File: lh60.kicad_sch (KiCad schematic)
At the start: 31 parts, among them J1 Conn_01x03_Female, J3 Conn_01x02_Female, J5 Conn_01x02_Female, P1 USB_C_Plug_USB2.0, SW1 SW_Push, U1 AMS1117-3.3, U2 STM32F103C8Tx, Y1 32.768K, Y2 8M

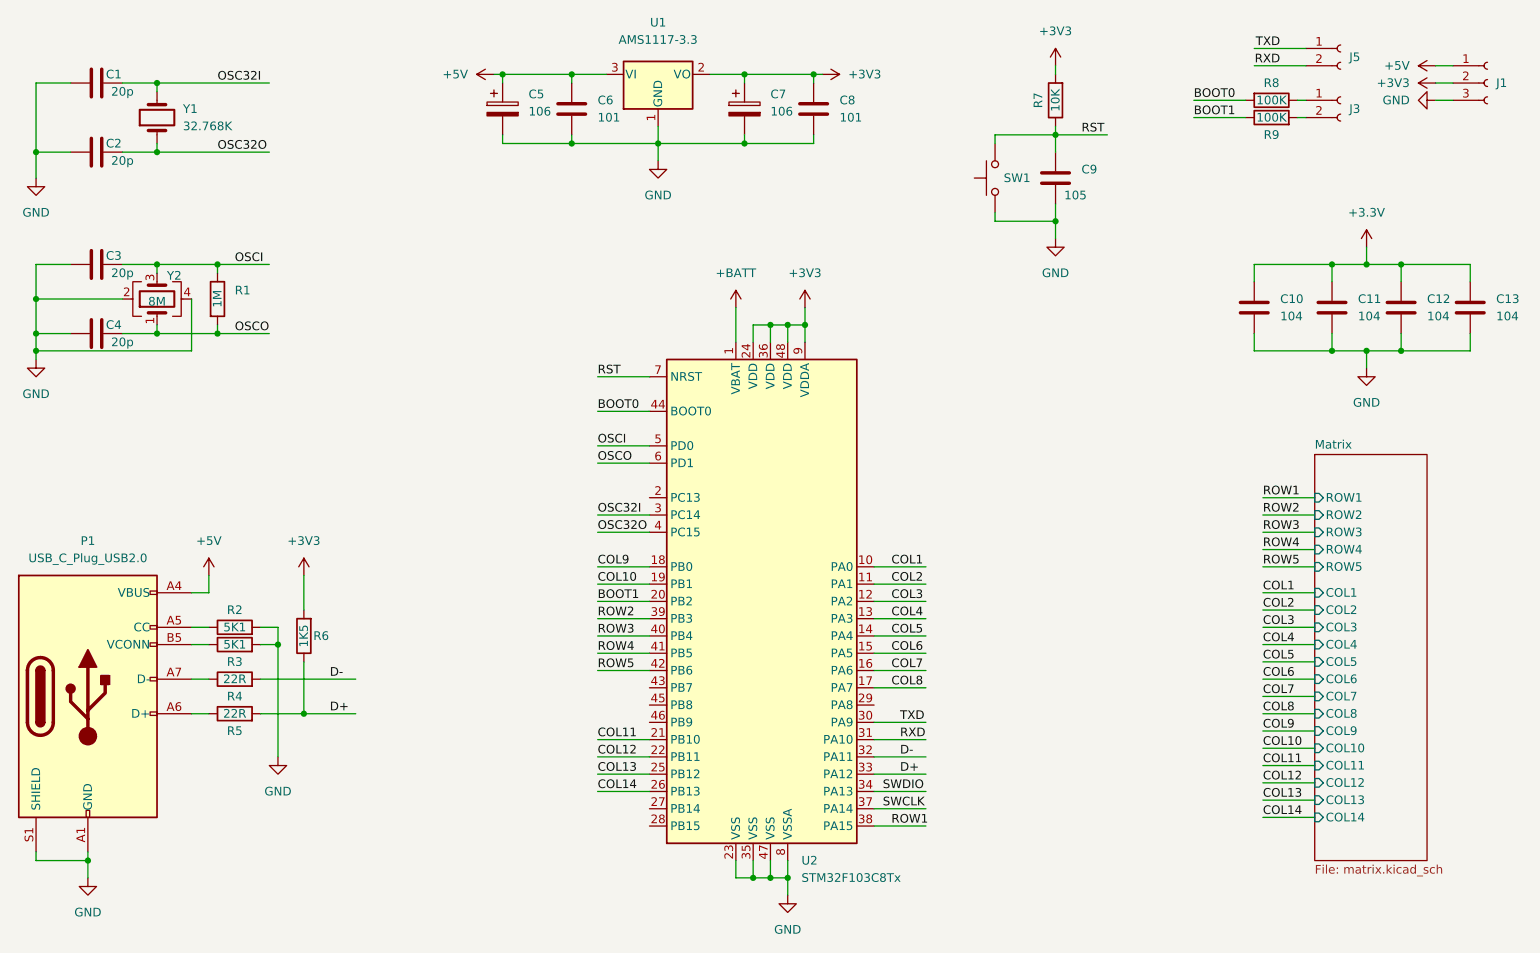
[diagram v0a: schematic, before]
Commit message: 20220401 sch 2.0
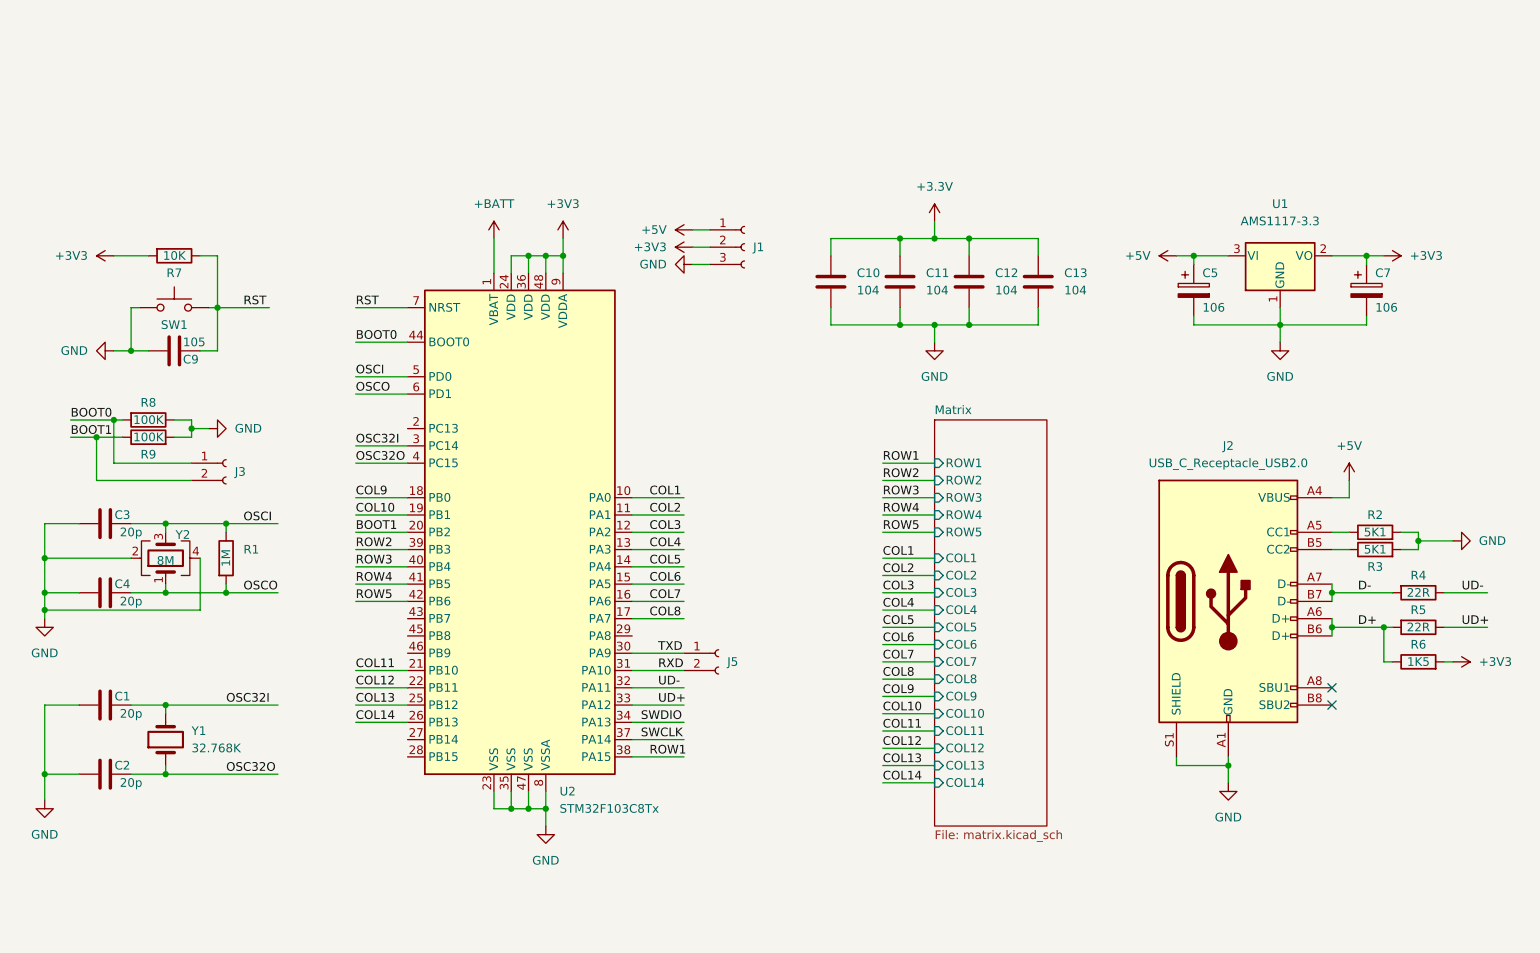
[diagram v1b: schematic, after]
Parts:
- removed C6, C8: 101, Capacitor_SMD:C_0603_1608Metric_Pad1.08x0.95mm_HandSolder, symbol Device:C
- removed P1: USB_C_Plug_USB2.0, Connector_USB:USB_C_Receptacle_HRO_TYPE-C-31-M-12, symbol Connector:USB_C_Plug_USB2.0
- added J2: USB_C_Receptacle_USB2.0, symbol Connector:USB_C_Receptacle_USB2.0
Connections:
- net +5V: now also J2.A4 (VBUS), J2.A9 (VBUS), J2.B4 (VBUS), J2.B9 (VBUS)
- net BOOT0: now also J3.1 (Pin_1)
- net BOOT1: now also J3.2 (Pin_2)
- net D+: now also J2.A6 (D+), J2.B6 (D+); no longer U2.33 (PA12)
- net D-: now also J2.A7 (D-), J2.B7 (D-); no longer U2.32 (PA11)
- net GND: now also R8.1, R9.2, J2.A1 (GND), J2.A12 (GND), J2.B1 (GND), J2.B12 (GND), J2.S1 (SHIELD)
- net at R2.1: now also J2.A5 (CC1)
- net UD-: now reaches R4.1
- net UD-: now also U2.32 (PA11)
- net UD+: now reaches R5.1
- net UD+: now also U2.33 (PA12)
- net at R3.1: now also J2.B5 (CC2)
- no-connect marks 0 -> 2
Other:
- moved on the sheet: C1, C10, C11, C12, C13, C2, C3, C4, C7, C9, J1, J3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
